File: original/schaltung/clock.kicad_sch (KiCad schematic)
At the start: 41 parts, among them K1 RESET, K2 MON, K3 MCYCL, K4 CYCL, Q1 7.3728M, T1 SS216

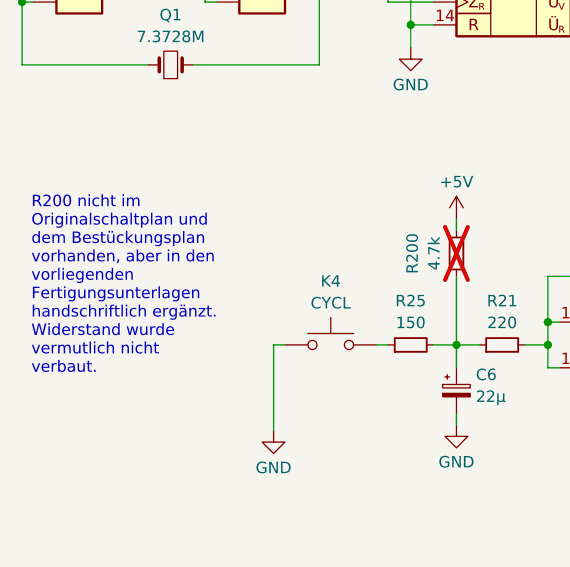
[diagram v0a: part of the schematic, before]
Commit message: Typo Schaltplan
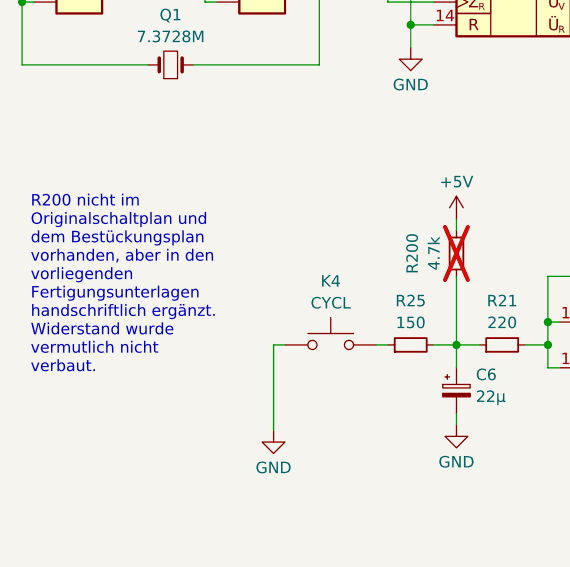
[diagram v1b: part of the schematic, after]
